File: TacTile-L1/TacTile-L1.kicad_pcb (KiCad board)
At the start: 2 copper layers, 2 parts, among them J1 Conn_01x02, J2 Conn_01x02

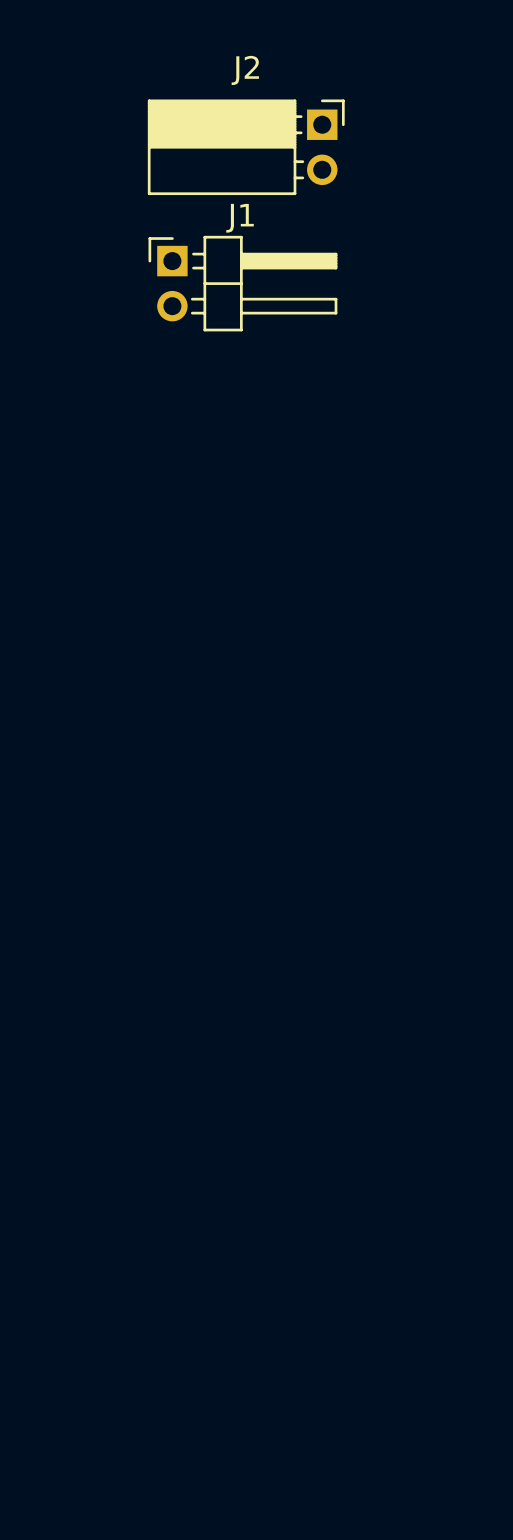
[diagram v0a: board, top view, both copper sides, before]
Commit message: Finished L1 Board
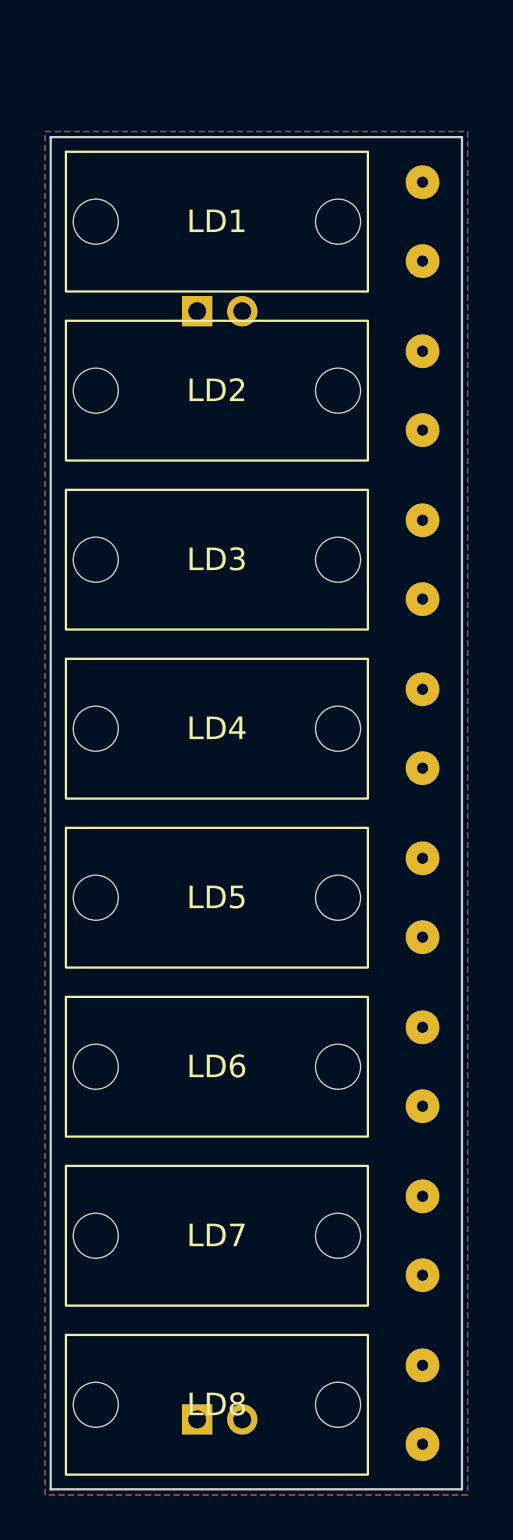
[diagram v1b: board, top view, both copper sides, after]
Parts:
- added LD1: D_Laser_1C2A, TacTile:Laser_Diode, F.Cu at (39.0, 28.8)
- added LD2: D_Laser_1C2A, TacTile:Laser_Diode, F.Cu at (39.0, 36.2)
- added LD3: D_Laser_1C2A, TacTile:Laser_Diode, F.Cu at (39.0, 43.8)
- added LD4: D_Laser_1C2A, TacTile:Laser_Diode, F.Cu at (39.0, 51.2)
- added LD5: D_Laser_1C2A, TacTile:Laser_Diode, F.Cu at (39.0, 58.8)
- added LD6: D_Laser_1C2A, TacTile:Laser_Diode, F.Cu at (39.0, 66.2)
- added LD7: D_Laser_1C2A, TacTile:Laser_Diode, F.Cu at (39.0, 73.8)
- added LD8: D_Laser_1C2A, TacTile:Laser_Diode, F.Cu at (39.0, 81.2)
- J1, J2: moved to B.Cu
- moved J1 51.4 mm to (31.5, 81.9), turned to -90 degrees
- moved J2 9.96 mm to (31.5, 32.7), turned to -90 degrees
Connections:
- J1 pad 1: Net-(J1-Pin_1) -> /VCC
- J1 pad 2: Net-(J1-Pin_2) -> /GND
- J2 pad 1: Net-(J1-Pin_2) -> /VCC
- J2 pad 2: Net-(J1-Pin_1) -> /GND
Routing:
- added copper zone on B.Cu, net /GND
- added copper zone on F.Cu, net /VCC
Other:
- board outline added: 18.2 x 60 mm
